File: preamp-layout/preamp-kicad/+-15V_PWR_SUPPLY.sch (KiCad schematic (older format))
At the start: 33 parts, among them J10 Conn_01x03_Male, J7 Screw_Terminal_01x03, J8 Conn_01x03_Male, J9 Conn_01x03_Male, T1 Transformer_1P_2S, U1 LM7815, U2 LM7915

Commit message: Periodic backup
Extensive changes as a result of PCB layout phase.
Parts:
- T1: footprint (none) -> preamp:164J28
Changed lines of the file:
@@
 F 0 "T1" H 2900 3939 50  0000 C CNN
 F 1 "Transformer_1P_2S" H 2900 3940 50  0001 C CNN
-F 2 "" H 2900 3450 50  0001 C CNN
+F 2 "preamp:164J28" H 2900 3450 50  0001 C CNN
 F 3 "~" H 2900 3450 50  0001 C CNN
 	1    2900 3450

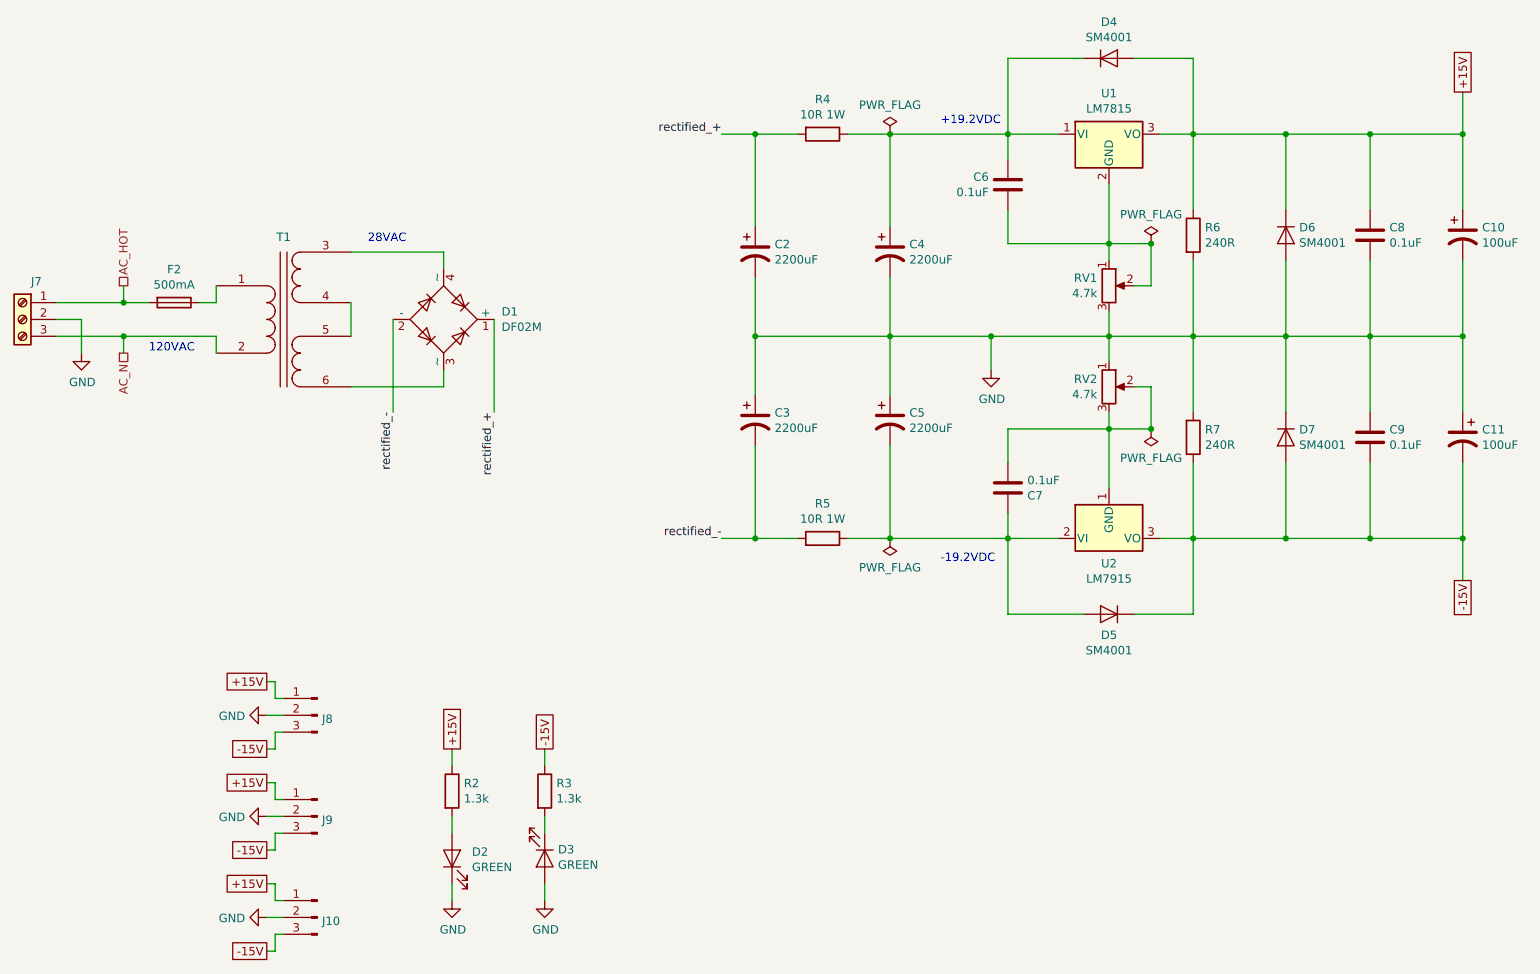
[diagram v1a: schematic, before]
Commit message: PCB layout
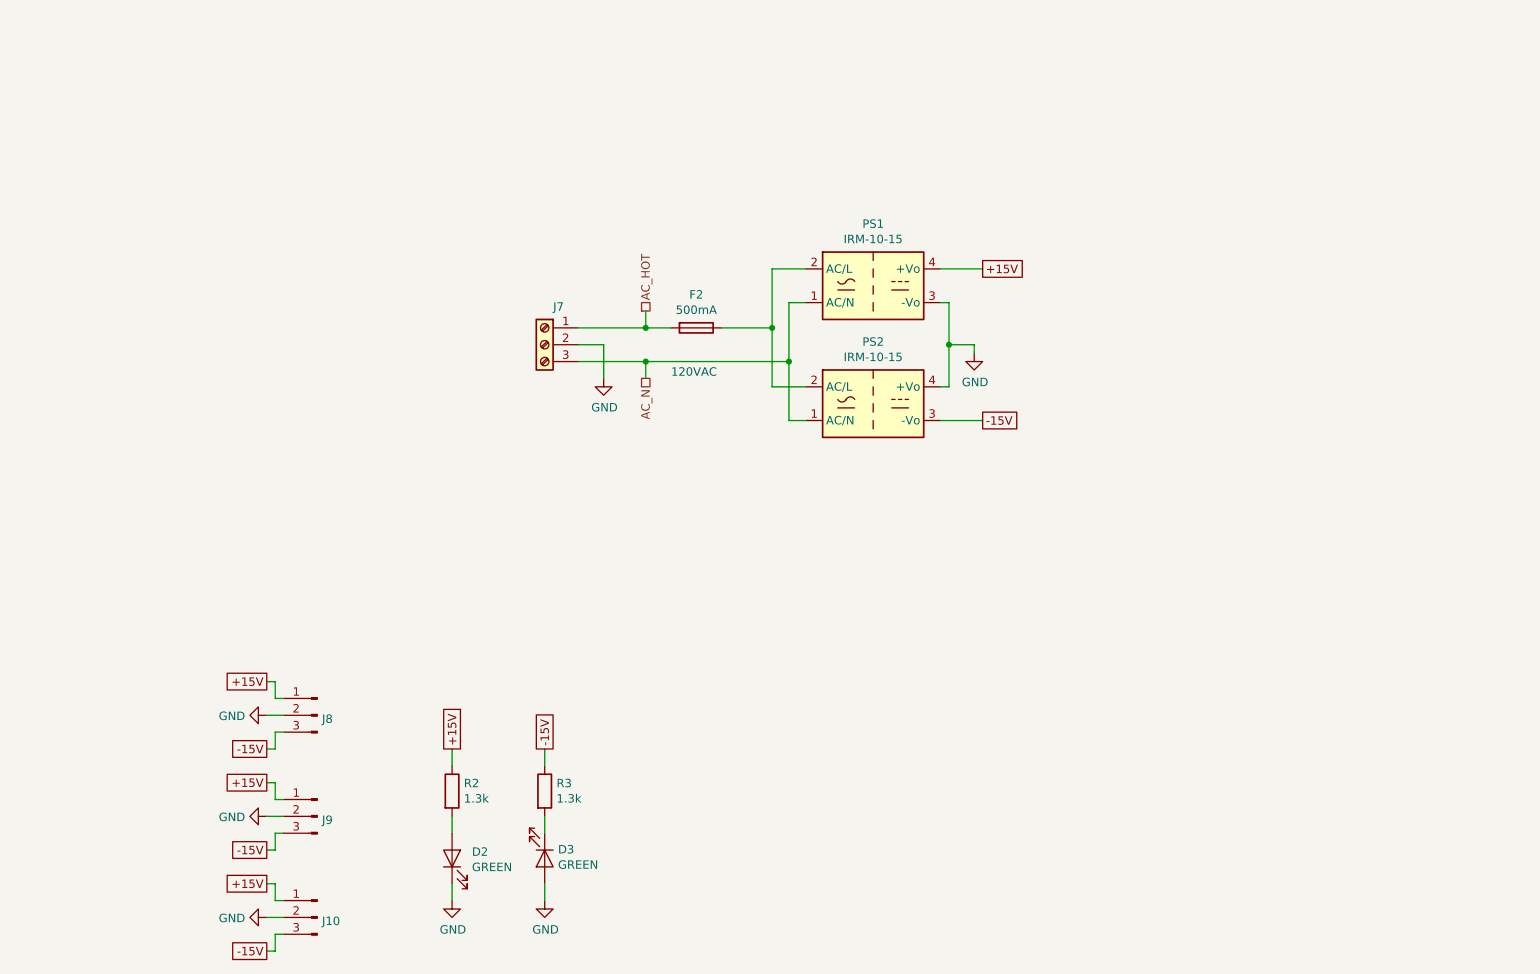
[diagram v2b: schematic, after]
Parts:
- removed C10, C11: 100uF, Capacitor_THT:CP_Radial_D6.3mm_P2.50mm, symbol Device:CP1
- removed C2, C3, C4, C5: 2200uF, Capacitor_THT:CP_Radial_D12.5mm_P5.00mm, symbol Device:CP1
- removed C6, C7, C8, C9: 0.1uF, Capacitor_SMD:C_0805_2012Metric_Pad1.15x1.40mm_HandSolder, symbol Device:C
- removed D1: DF02M, Diode_THT:Diode_Bridge_DIP-4_W7.62mm_P5.08mm, symbol Diode_Bridge:DF02M
- removed D4, D5, D6, D7: SM4001, Diode_SMD:D_SOD-123F, symbol Device:D
- removed R4, R5: 10R 1W, Resistor_THT:R_Axial_DIN0414_L11.9mm_D4.5mm_P15.24mm_Horizontal, symbol Device:R
- removed R6, R7: 240R, Resistor_SMD:R_1206_3216Metric_Pad1.42x1.75mm_HandSolder, symbol Device:R
- removed RV1, RV2: 4.7k, Potentiometer_THT:Potentiometer_Bourns_3386P_Vertical, symbol Device:R_POT
- removed T1: Transformer_1P_2S, preamp:164J28, symbol Device:Transformer_1P_2S
- removed U1: LM7815, Package_TO_SOT_THT:TO-220-3_Vertical, symbol Regulator_Linear:LM7815_TO220
- removed U2: LM7915, Package_TO_SOT_THT:TO-220-3_Vertical, symbol Regulator_Linear:LM7915_TO220
- added PS1, PS2: IRM-10-15, Converter_ACDC:Converter_ACDC_MeanWell_IRM-10-xx_THT, symbol Converter_ACDC:IRM-10-15
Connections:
- net +15V: now also PS1.4 (+Vo)
- net -15V: now also PS2.3 (-Vo)
- net AC_N: now also PS1.1 (AC/N), PS2.1 (AC/N)
- net GND: now also PS1.3 (-Vo), PS2.4 (+Vo)
- net at F2.1: now also PS1.2 (AC/L), PS2.2 (AC/L)
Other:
- note removed: "+19.2VDC"
- note removed: "-19.2VDC"
- note removed: "28VAC"
- moved on the sheet: F2, J7
